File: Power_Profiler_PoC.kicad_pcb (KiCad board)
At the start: 2 copper layers, 8 parts, among them J1 Conn_01x05_Pin, J2 Conn_01x05_Socket, J3 Screw_Terminal_01x02, U1 LTC2944IDD#PBF

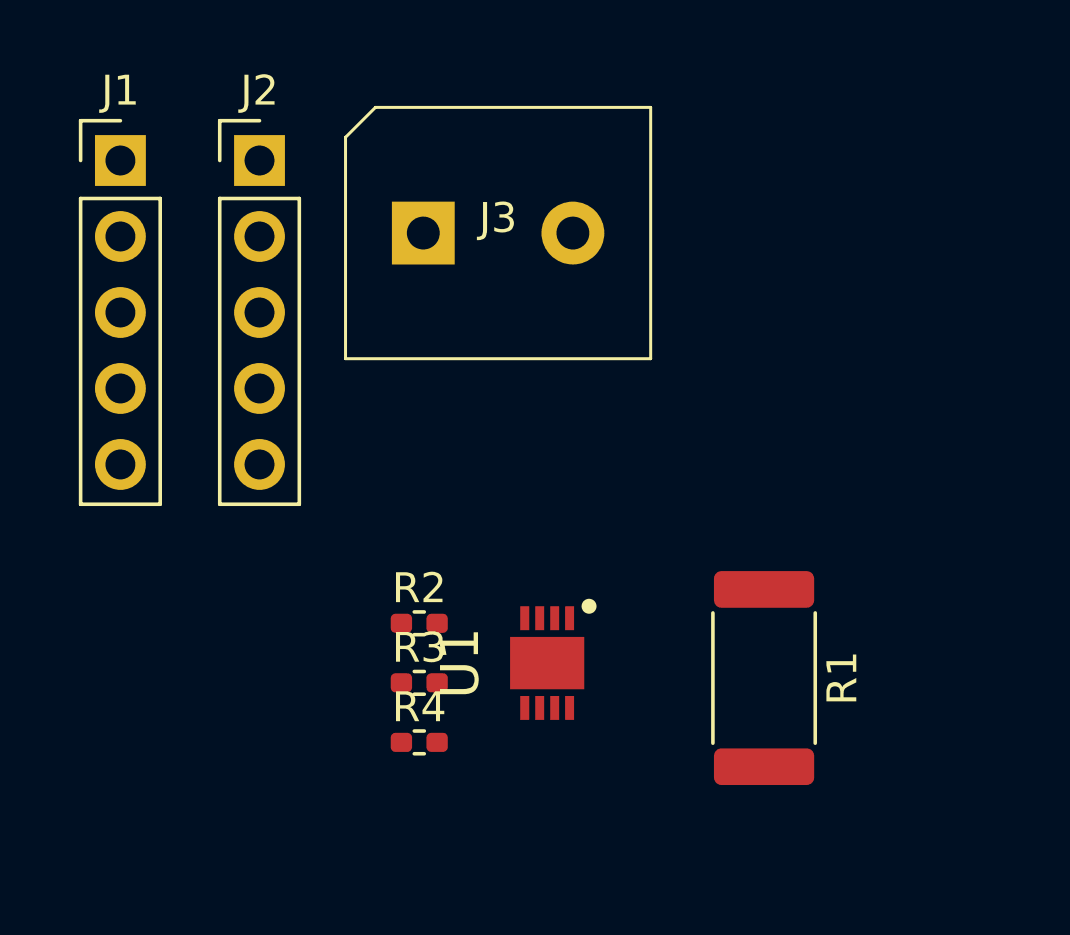
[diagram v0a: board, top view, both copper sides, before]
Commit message: Started routing
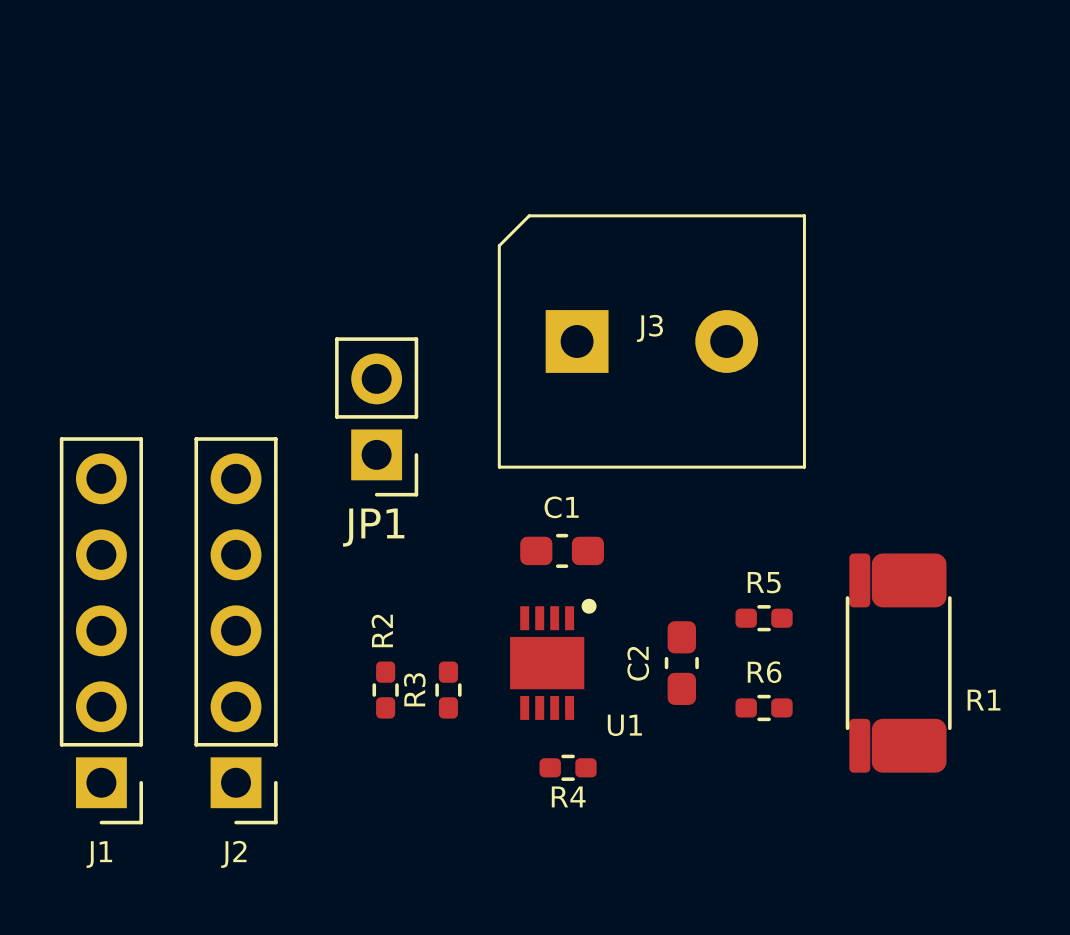
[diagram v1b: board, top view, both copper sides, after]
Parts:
- added C1: 1uF, PP_PoC:C_0603_1608Metric_Pad1.08x0.95mm_HandSolder, F.Cu at (154.5, 101.8)
- added C2: 100nF, PP_PoC:C_0603_1608Metric_Pad1.08x0.95mm_HandSolder, F.Cu at (158.5, 105.5)
- added JP1: Jumper_2_Open, PP_PoC:PinHeader_1x02_P2.54mm_Vertical, F.Cu at (148.3, 98.5)
- added R5: 100E, PP_PoC:R_0402_1005Metric_Pad0.72x0.64mm_HandSolder, F.Cu at (161.2, 104.0)
- added R6: 100E, PP_PoC:R_0402_1005Metric_Pad0.72x0.64mm_HandSolder, F.Cu at (161.2, 107.0)
- R2, R3, R4: value 2k2 -> 2k
- moved J2 20.8 mm to (143.6, 109.5), turned to 180 degrees
- moved J1 20.8 mm to (139.1, 109.5), turned to 180 degrees
- moved J3 6.29 mm to (157.5, 94.8)
- moved R4 5.05 mm to (154.7, 109.0), turned to 180 degrees
- moved R1 4.53 mm to (165.8, 105.5)
- moved R2 2.50 mm to (148.6, 106.4), turned to -90 degrees
- moved R3 1.00 mm to (150.7, 106.4), turned to -90 degrees
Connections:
- J1 pad 1: /Ext_Connector/3V3 -> /SCL
- J1 pad 2: GND -> /SDA
- J1 pad 3: /Ext_Connector/~{ALCC} -> /~{ALCC}
- J1 pad 4: /Ext_Connector/MCU_SDA -> /3V3/5V
- J1 pad 5: /Ext_Connector/MCU_SCL -> GND
- J2 pad 1: /Ext_Connector/3V3 -> /SCL
- J2 pad 2: GND -> /SDA
- J2 pad 3: /Ext_Connector/~{ALCC} -> /~{ALCC}
- J2 pad 4: /Ext_Connector/MCU_SDA -> /3V3/5V
- J2 pad 5: /Ext_Connector/MCU_SCL -> GND
- R1 pad 1: /SHUNT/BATT+_OUT -> GND
- R1 pad 2: /SHUNT/SENSE-_OUT -> Net-(R1-Pad2)
- R2 pad 1: /LTC2944/3V3 -> /3V3/5V
- R2 pad 2: /LTC2944/MCU_SDA -> /SCL
- R3 pad 1: /LTC2944/3V3 -> /3V3/5V
- R3 pad 2: /LTC2944/MCU_SCL -> /SDA
- R4 pad 1: /LTC2944/3V3 -> /3V3/5V
- R4 pad 2: /LTC2944/~{ALCC} -> /~{ALCC}
- U1 pad 4: /LTC2944/MCU_SCL -> /SCL
- U1 pad 5: /LTC2944/MCU_SDA -> /SDA
- U1 pad 6: /LTC2944/~{ALCC} -> /~{ALCC}
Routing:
- net /3V3/5V: track 0.00 -> 0.71 mm
